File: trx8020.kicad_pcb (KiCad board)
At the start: 2 copper layers, 12 parts, among them IC1 NE5534, IC2 78L10, M1 Mic

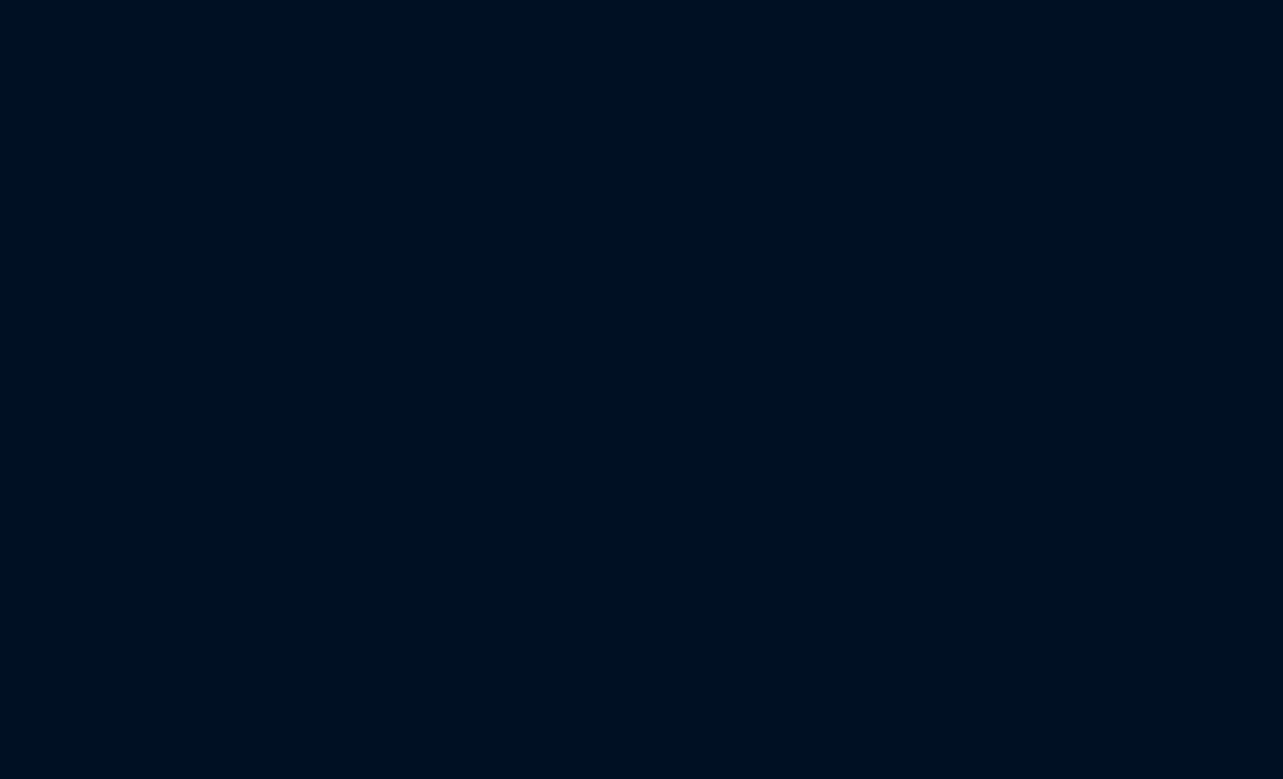
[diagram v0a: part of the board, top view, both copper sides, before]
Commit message: ...
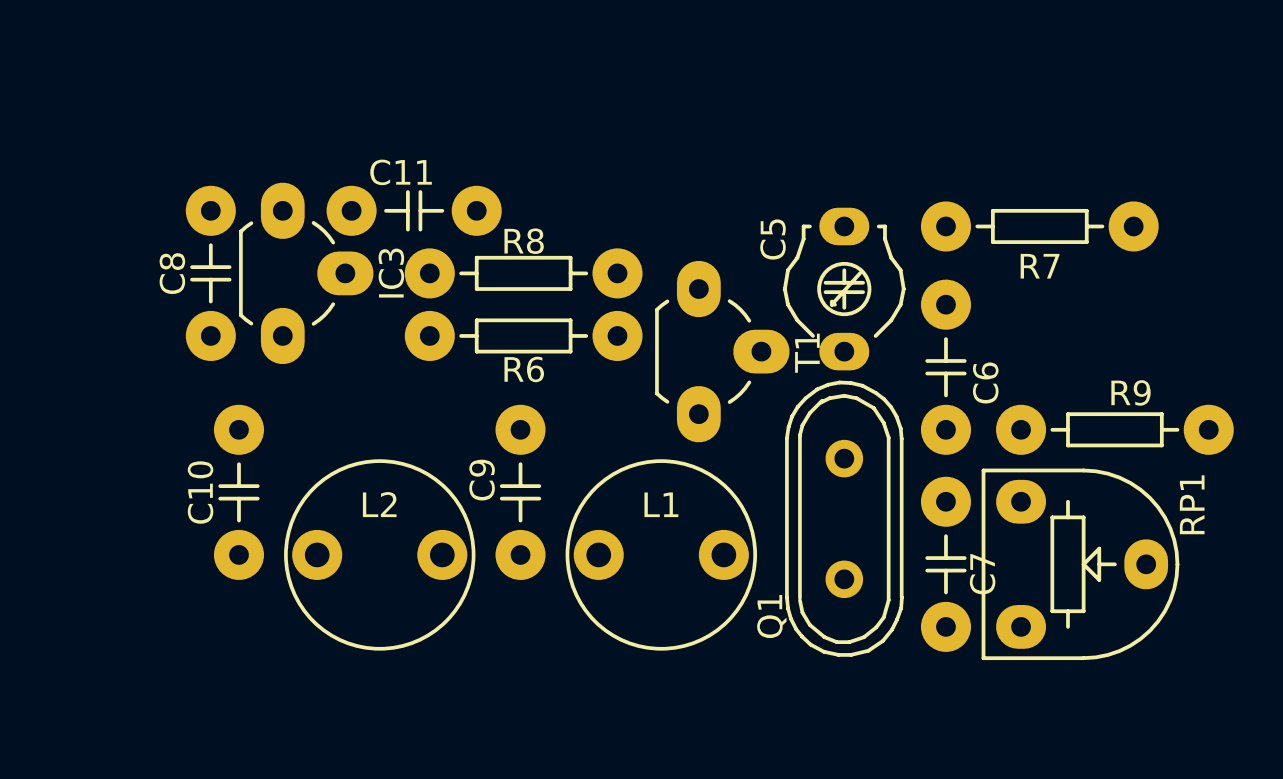
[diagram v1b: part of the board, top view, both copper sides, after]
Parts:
- added C10: Capacitor, Raberix:C2, F.Cu at (76.3, 183.4)
- added C11: 100n, Raberix:C2, F.Cu at (83.4, 172.0)
- added C5: 6-22p, Raberix:C2Trim, F.Cu at (100.9, 177.7)
- added C6: 220p, Raberix:C2, F.Cu at (105.0, 178.3)
- added C7: 220p, Raberix:C2, F.Cu at (105.0, 186.3)
- added C8: 100n, Raberix:C2, F.Cu at (75.2, 174.5)
- added C9: Capacitor, Raberix:C2, F.Cu at (87.8, 183.4)
- added IC3: 78Lxx, Raberix:TO-92, F.Cu at (78.1, 172.0)
- added L1: 47u, Raberix:Inductor, F.Cu at (93.5, 185.9)
- added L2: 47u, Raberix:Inductor, F.Cu at (82.0, 185.9)
- added Q1: 6 MHz, Raberix:HC49-U, F.Cu at (100.9, 184.5)
- added R6: 100k, Raberix:R3, F.Cu at (87.9, 177.0)
- added R7: 680k, Raberix:R3, F.Cu at (108.8, 172.6)
- added R8: 100, Raberix:R3, F.Cu at (87.9, 174.5)
- added R9: 1k, Raberix:R3, F.Cu at (111.9, 180.8)
- added RP1: 10k, Raberix:RM-065, F.Cu at (108.1, 186.3)
- added T1: BC-547, Raberix:TO-92, F.Cu at (95.0, 175.1)

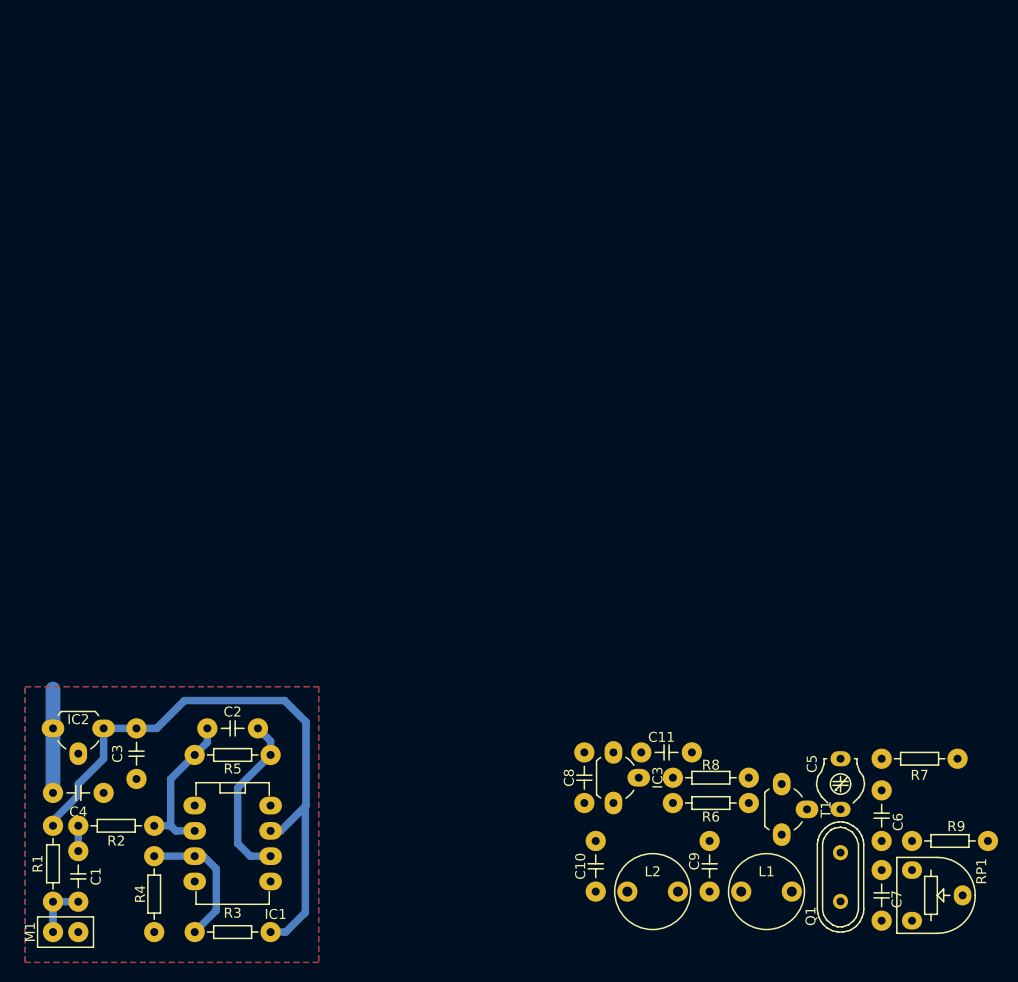
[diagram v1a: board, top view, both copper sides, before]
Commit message: ...
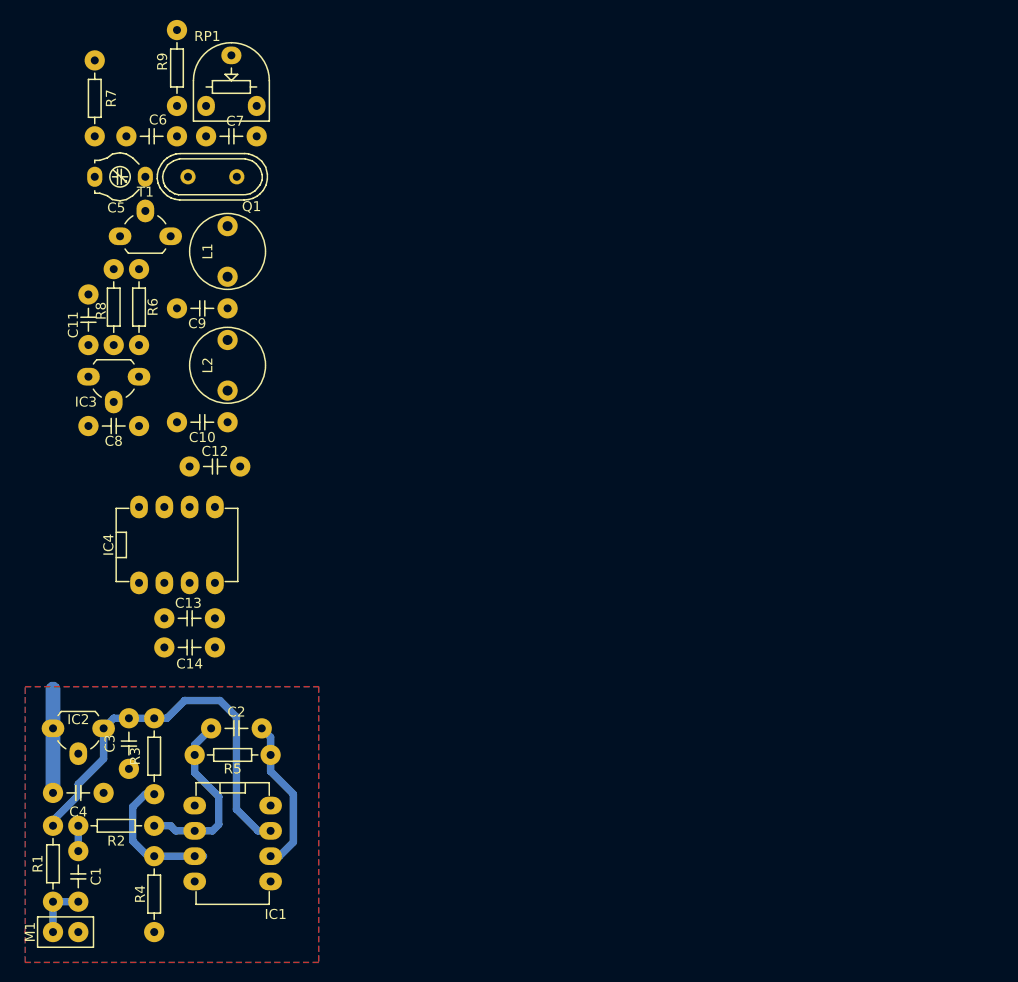
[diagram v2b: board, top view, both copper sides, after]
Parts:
- added C12: 100n, Raberix:C2, F.Cu at (38.1, 143.3)
- added C13: 1u, Raberix:C2, F.Cu at (35.6, 158.5)
- added C14: 1u, Raberix:C2, F.Cu at (35.6, 161.4)
- added IC4: SA612, Raberix:DIP-8, F.Cu at (30.5, 154.9)
- C10: value Capacitor -> 10p
- C9: value Capacitor -> 33p
- IC3: value 78Lxx -> 78L06
- moved R9 109.7 mm to (34.3, 103.3), turned to 90 degrees
- moved R7 106.1 mm to (26.0, 106.3), turned to 90 degrees
- moved RP1 104.6 mm to (39.8, 107.1), turned to 180 degrees
- moved C7 100.3 mm to (39.8, 110.1), turned to 0 degrees
- moved C6 100.1 mm to (31.8, 110.1), turned to 0 degrees
- moved Q1 94.4 mm to (37.8, 114.2), turned to 180 degrees
- moved C5 94.4 mm to (31.1, 114.2), turned to 270 degrees
- moved T1 86.2 mm to (28.6, 120.1), turned to 0 degrees
- moved L1 84.0 mm to (39.4, 121.7), turned to 270 degrees
- moved R8 76.3 mm to (27.9, 127.3), turned to 90 degrees
- moved R6 76.0 mm to (30.5, 127.3), turned to 90 degrees
- moved C9 75.7 mm to (36.8, 127.4), turned to 180 degrees
- moved C11 72.5 mm to (25.4, 128.5), turned to 90 degrees
- moved L2 67.9 mm to (39.4, 133.1), turned to 270 degrees
- moved IC3 60.8 mm to (30.5, 134.2), turned to 180 degrees
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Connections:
- IC3 pad 1: Net-(C11-Pad2) -> Net-(C8-Pad2)
- IC3 pad 3: Net-(C8-Pad2) -> Net-(C11-Pad2)
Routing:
- net Net-(C3-Pad2): track 63.2 -> 40.7 mm
- net Net-(C2-Pad2): track 15.6 -> 18.3 mm
- net Net-(C14-Pad1): track 17.3 -> 15.6 mm
